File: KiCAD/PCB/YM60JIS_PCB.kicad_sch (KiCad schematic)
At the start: 165 parts, among them J1 TYPE-C-31-M-12, SW1 SW_Push, SW10 SW_Push, SW11 SW_Push, SW12 SW_Push, SW13 SW_Push, SW14 SW_Push, SW15 SW_Push, SW16 SW_Push, SW17 SW_Push, SW18 SW_Push, SW19 SW_Push, SW2 SW_Push, SW20 SW_Push, SW21 SW_Push, SW22 SW_Push, SW23 SW_Push, SW24 SW_Push, SW25 SW_Push, SW26 SW_Push, SW27 SW_Push, SW28 SW_Push, SW29 Space, SW3 SW_Push, SW30 SW_Push, SW31 SW_Push, SW32 SW_Push, SW33 SW_Push, SW34 SW_Push, SW35 SW_Push, SW36 SW_Push, SW37 SW_Push, SW38 SW_Push, SW39 SW_Push, SW4 SW_Push, SW40 SW_Push, SW41 SW_Push, SW42 SW_Push, SW43 SW_Push, SW44 SW_Push, SW45 SW_Push, SW46 SW_Push, SW47 SW_Push, SW48 SW_Push, SW49 SW_Push, SW5 SW_Push, SW50 SW_Push, SW51 SW_Push, SW52 SW_Push, SW53 SW_Push, SW54 SW_Push, SW55 SW_Push, SW56 SW_Push, SW57 SW_Push, SW58 SW_Push, SW59 SW_Push, SW6 SW_Push, SW60 SW_Push, SW61 SW_Push, SW62 SW_Push, SW63 Yen, SW64 Backspace, SW65 ISOEnter, SW66 SW_Push, SW67 SW_Push, SW7 SW_Push, SW8 SW_Push, SW9 SW_Push, U1 XC6206P332MR, U2 SMF05CT1G, U3 RP2040, U4 W25Q16JVUXIQ, Y1 X322512MSB4SI

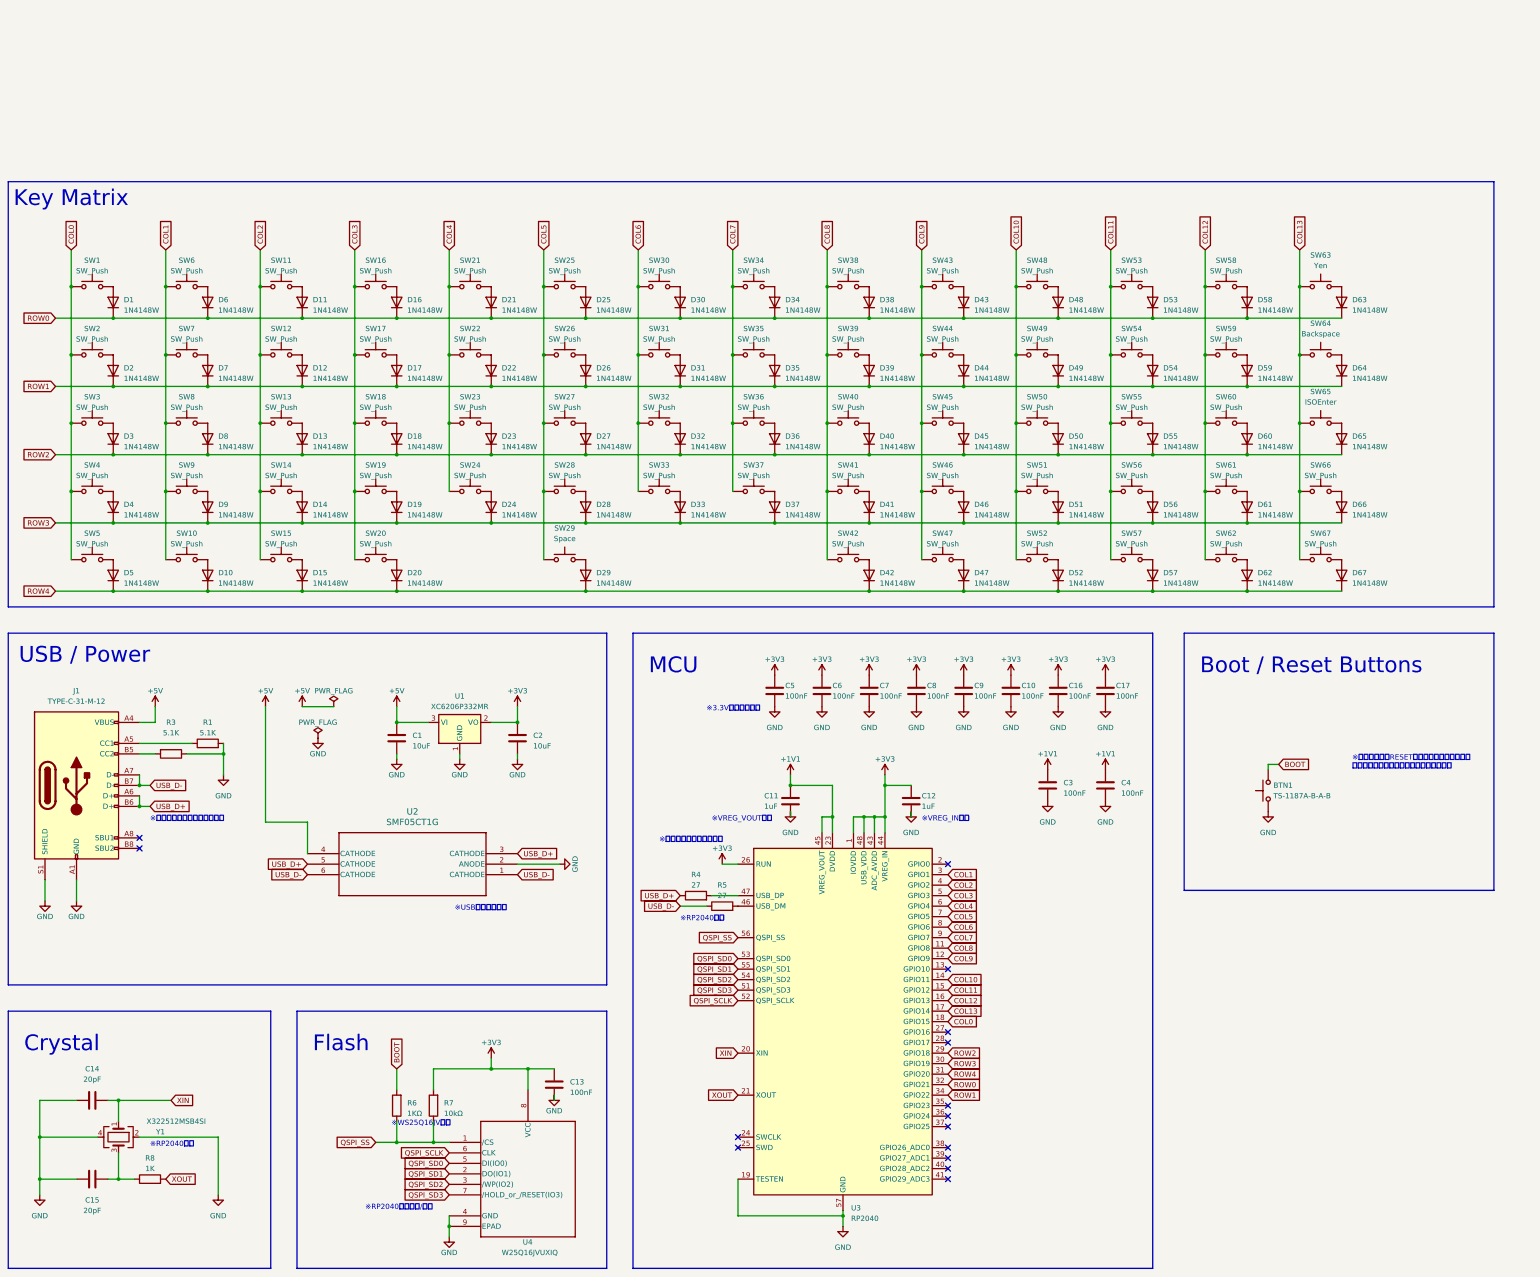
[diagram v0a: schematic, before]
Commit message: reroute
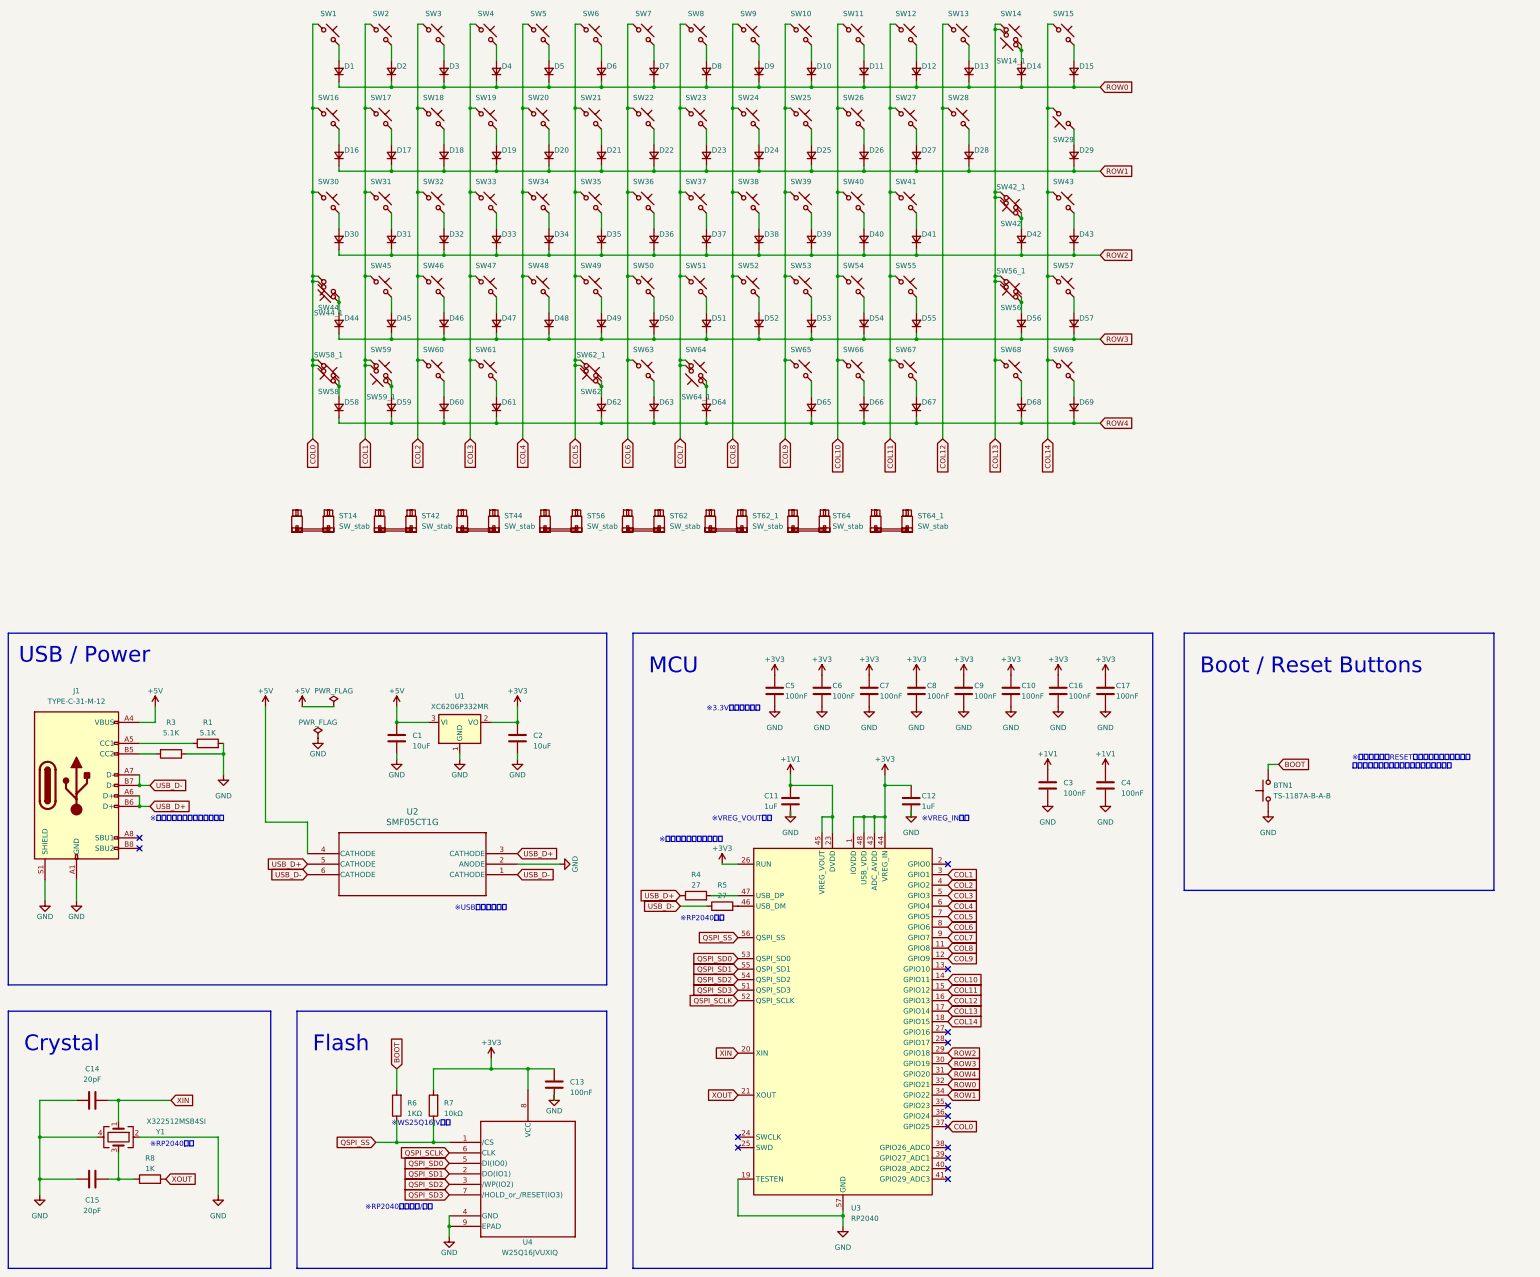
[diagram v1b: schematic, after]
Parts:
- removed D1, D10, D11, D12, D13, D14, D15, D16, D17, D18, D19, D2, D20, D21, D22, D23, D24, D25, D26, D27, D28, D29, D3, D30, D31, D32, D33, D34, D35, D36, D37, D38, D39, D4, D40, D41, D42, D43, D44, D45, D46, D47, D48, D49, D5, D50, D51, D52, D53, D54, D55, D56, D57, D58, D59, D6, D60, D61, D62, D63, D64, D65, D66, D67, D7, D8, D9: 1N4148W, Diode_SMD:D_SOD-123, symbol Diode:1N4148W
- removed SW1, SW11, SW12, SW13, SW14, SW16, SW17, SW18, SW19, SW21, SW22, SW23, SW24, SW25, SW26, SW27, SW28, SW30, SW31, SW32, SW33, SW34, SW35, SW36, SW37, SW38, SW39, SW4, SW40, SW41, SW42, SW43, SW44, SW45, SW46, SW48, SW49, SW50, SW51, SW53, SW54, SW55, SW56, SW57, SW58, SW59, SW6, SW60, SW61, SW62, SW66, SW67, SW7, SW8, SW9: SW_Push, PCM_marbastlib-mx:SW_MX_HS_CPG151101S11_1u, symbol Switch:SW_Push
- removed SW10, SW15, SW20, SW47, SW52: SW_Push, PCM_marbastlib-mx:SW_MX_HS_CPG151101S11_1.25u, symbol Switch:SW_Push
- removed SW2, SW5: SW_Push, PCM_marbastlib-mx:SW_MX_HS_CPG151101S11_1.5u, symbol Switch:SW_Push
- removed SW29: Space, PCM_marbastlib-mx:SW_MX_HS_CPG151101S11_1u, symbol Switch:SW_Push
- removed SW3: SW_Push, PCM_marbastlib-mx:SW_MX_HS_CPG151101S11_1.75u, symbol Switch:SW_Push
- removed SW63: Yen, PCM_marbastlib-mx:SW_MX_HS_CPG151101S11_1u, symbol Switch:SW_Push
- removed SW64: Backspace, PCM_marbastlib-mx:SW_MX_HS_CPG151101S11_1u, symbol Switch:SW_Push
- removed SW65: ISOEnter, PCM_marbastlib-mx:SW_MX_HS_CPG151101S11_1u, symbol Switch:SW_Push
- added D1, D10, D11, D12, D13, D14, D15, D16, D17, D18, D19, D2, D20, D21, D22, D23, D24, D25, D26, D27, D28, D29, D3, D30, D31, D32, D33, D34, D35, D36, D37, D38, D39, D4, D40, D41, D42, D43, D44, D45, D46, D47, D48, D49, D5, D50, D51, D52, D53, D54, D55, D56, D57, D58, D59, D6, D60, D61, D62, D63, D64, D65, D66, D67, D68, D69, D7, D8, D9: D, Diode_SMD:D_SOD-123, symbol Device:D_Small
- added ST14, ST42, ST44, ST56, ST62, ST62_1, ST64, ST64_1: SW_stab, PCM_marbastlib-mx:STAB_MX_2u, symbol Mechanical:SW_stab
- added SW1, SW10, SW11, SW12, SW13, SW14, SW14_1, SW15, SW17, SW18, SW19, SW2, SW20, SW21, SW22, SW23, SW24, SW25, SW26, SW27, SW28, SW3, SW31, SW32, SW33, SW34, SW35, SW36, SW37, SW38, SW39, SW4, SW40, SW41, SW42, SW43, SW44, SW44_1, SW46, SW47, SW48, SW49, SW5, SW50, SW51, SW52, SW53, SW54, SW55, SW56, SW57, SW58_1, SW59, SW6, SW60, SW61, SW62, SW62_1, SW63, SW64, SW64_1, SW65, SW66, SW7, SW8, SW9: SW_Push, PCM_marbastlib-mx:SW_MX_HS_CPG151101S11_1u, symbol Switch:SW_Push_45deg
- added SW16, SW29: SW_Push, PCM_marbastlib-mx:SW_MX_HS_CPG151101S11_1.5u, symbol Switch:SW_Push_45deg
- added SW30, SW56_1: SW_Push, PCM_marbastlib-mx:SW_MX_HS_CPG151101S11_1.75u, symbol Switch:SW_Push_45deg
- added SW42_1, SW45, SW58, SW59_1, SW67, SW68, SW69: SW_Push, PCM_marbastlib-mx:SW_MX_HS_CPG151101S11_1.25u, symbol Switch:SW_Push_45deg
- U2: footprint SOT-363-6_2P2X1P35_ONS -> SMF05CT1G:SOT-363-6_2P2X1P35_ONS
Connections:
- net COL0: now also U3.37 (GPIO25), SW1.1, SW16.1, SW30.1, SW44.2, SW44_1.2, SW58.2, SW58_1.1; no longer U3.18 (GPIO15)
- net COL1: now also SW17.1, SW2.1, SW31.1, SW45.1, SW59.1, SW59_1.2
- net COL10: now also SW11.1, SW26.1, SW40.1, SW54.1, SW66.1
- net COL11: now also SW12.1, SW27.1, SW41.1, SW55.1, SW67.1
- net COL12: now also SW13.1, SW28.1
- net COL13: now also SW14.1, SW14_1.2, SW42.2, SW42_1.1, SW56.2, SW56_1.1, SW68.1
- net COL2: now also SW18.1, SW3.1, SW32.1, SW46.1, SW60.1
- net COL3: now also SW19.1, SW33.1, SW4.1, SW47.1, SW61.1
- net COL4: now also SW20.1, SW34.1, SW48.1, SW5.1
- net COL5: now also SW21.1, SW35.1, SW49.1, SW6.1, SW62.2, SW62_1.1
- net COL6: now also SW22.1, SW36.1, SW50.1, SW63.1, SW7.1
- net COL7: now also SW23.1, SW37.1, SW51.1, SW64.1, SW64_1.2, SW8.1
- net COL8: now also SW24.1, SW38.1, SW52.1, SW9.1
- net COL9: now also SW10.1, SW25.1, SW39.1, SW53.1, SW65.1
- net ROW0: now also D1.1 (K), D10.1 (K), D11.1 (K), D12.1 (K), D13.1 (K), D14.1 (K), D15.1 (K), D2.1 (K), D3.1 (K), D4.1 (K), D5.1 (K), D6.1 (K), D7.1 (K), D8.1 (K), D9.1 (K)
- net ROW1: now also D16.1 (K), D17.1 (K), D18.1 (K), D19.1 (K), D20.1 (K), D21.1 (K), D22.1 (K), D23.1 (K), D24.1 (K), D25.1 (K), D26.1 (K), D27.1 (K), D28.1 (K), D29.1 (K)
- net ROW2: now also D30.1 (K), D31.1 (K), D32.1 (K), D33.1 (K), D34.1 (K), D35.1 (K), D36.1 (K), D37.1 (K), D38.1 (K), D39.1 (K), D40.1 (K), D41.1 (K), D42.1 (K), D43.1 (K)
- net ROW3: now also D44.1 (K), D45.1 (K), D46.1 (K), D47.1 (K), D48.1 (K), D49.1 (K), D50.1 (K), D51.1 (K), D52.1 (K), D53.1 (K), D54.1 (K), D55.1 (K), D56.1 (K), D57.1 (K)
- net ROW4: now also D58.1 (K), D59.1 (K), D60.1 (K), D61.1 (K), D62.1 (K), D63.1 (K), D64.1 (K), D65.1 (K), D66.1 (K), D67.1 (K), D68.1 (K), D69.1 (K)
- new net: D48.2 (A), SW48.2
- new net: D58.2 (A), SW58.1, SW58_1.2
- new net: D59.2 (A), SW59.2, SW59_1.1
- new net: D67.2 (A), SW67.2
- new net: D56.2 (A), SW56.1, SW56_1.2
- new net: D31.2 (A), SW31.2
- new net: D32.2 (A), SW32.2
- new net: D9.2 (A), SW9.2
- new net: D46.2 (A), SW46.2
- new net: D28.2 (A), SW28.2
- new net: D21.2 (A), SW21.2
- new net: D66.2 (A), SW66.2
- new net: D65.2 (A), SW65.2
- new net: D55.2 (A), SW55.2
- new net: D35.2 (A), SW35.2
- new net: D37.2 (A), SW37.2
- new net: D25.2 (A), SW25.2
- new net: D42.2 (A), SW42.1, SW42_1.2
- new net: D16.2 (A), SW16.2
- new net: D13.2 (A), SW13.2
- new net: D8.2 (A), SW8.2
- new net: D5.2 (A), SW5.2
- new net: D14.2 (A), SW14.2, SW14_1.1
- new net: D22.2 (A), SW22.2
- new net: D11.2 (A), SW11.2
- new net: D15.2 (A), SW15.2
- new net: D1.2 (A), SW1.2
- new net: D52.2 (A), SW52.2
- new net: D17.2 (A), SW17.2
- new net: D69.2 (A), SW69.2
- new net: D24.2 (A), SW24.2
- new net: D29.2 (A), SW29.1
- new net: D40.2 (A), SW40.2
- new net: D19.2 (A), SW19.2
- new net: D68.2 (A), SW68.2
- new net: D62.2 (A), SW62.1, SW62_1.2
- new net: D30.2 (A), SW30.2
- new net: D61.2 (A), SW61.2
- new net: D43.2 (A), SW43.2
- new net: D10.2 (A), SW10.2
- new net: D57.2 (A), SW57.2
- new net: D41.2 (A), SW41.2
- new net: D38.2 (A), SW38.2
- new net: D2.2 (A), SW2.2
- new net: D60.2 (A), SW60.2
- new net: D50.2 (A), SW50.2
- new net: D36.2 (A), SW36.2
- new net: D47.2 (A), SW47.2
- new net: D7.2 (A), SW7.2
- new net: D39.2 (A), SW39.2
- new net: D18.2 (A), SW18.2
- new net: D49.2 (A), SW49.2
- new net: D53.2 (A), SW53.2
- new net: D4.2 (A), SW4.2
- new net: D45.2 (A), SW45.2
- new net: D12.2 (A), SW12.2
- new net: D33.2 (A), SW33.2
- new net: D34.2 (A), SW34.2
- new net: D20.2 (A), SW20.2
- new net: D6.2 (A), SW6.2
- new net: D64.2 (A), SW64.2, SW64_1.1
- new net: D54.2 (A), SW54.2
- new net: D27.2 (A), SW27.2
- new net: D23.2 (A), SW23.2
- new net: D63.2 (A), SW63.2
- new net: D26.2 (A), SW26.2
- new net: D3.2 (A), SW3.2
- new net: D44.2 (A), SW44.1, SW44_1.1
- new net: D51.2 (A), SW51.2
- new net COL14: SW15.1, SW29.2, SW43.1, SW57.1, SW69.1, U3.18 (GPIO15)
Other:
- note removed: "Key Matrix"
